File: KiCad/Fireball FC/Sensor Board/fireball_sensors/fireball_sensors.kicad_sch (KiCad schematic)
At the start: 28 parts, among them CN1 HDGC2001WR-S-2P, J1 Conn_01x07, SW2 MAIN POWER, U2 MAX17048G, U3 TPS61023, U5 NCP708, U8 LSM6DSO, U9 MS5607-02BA

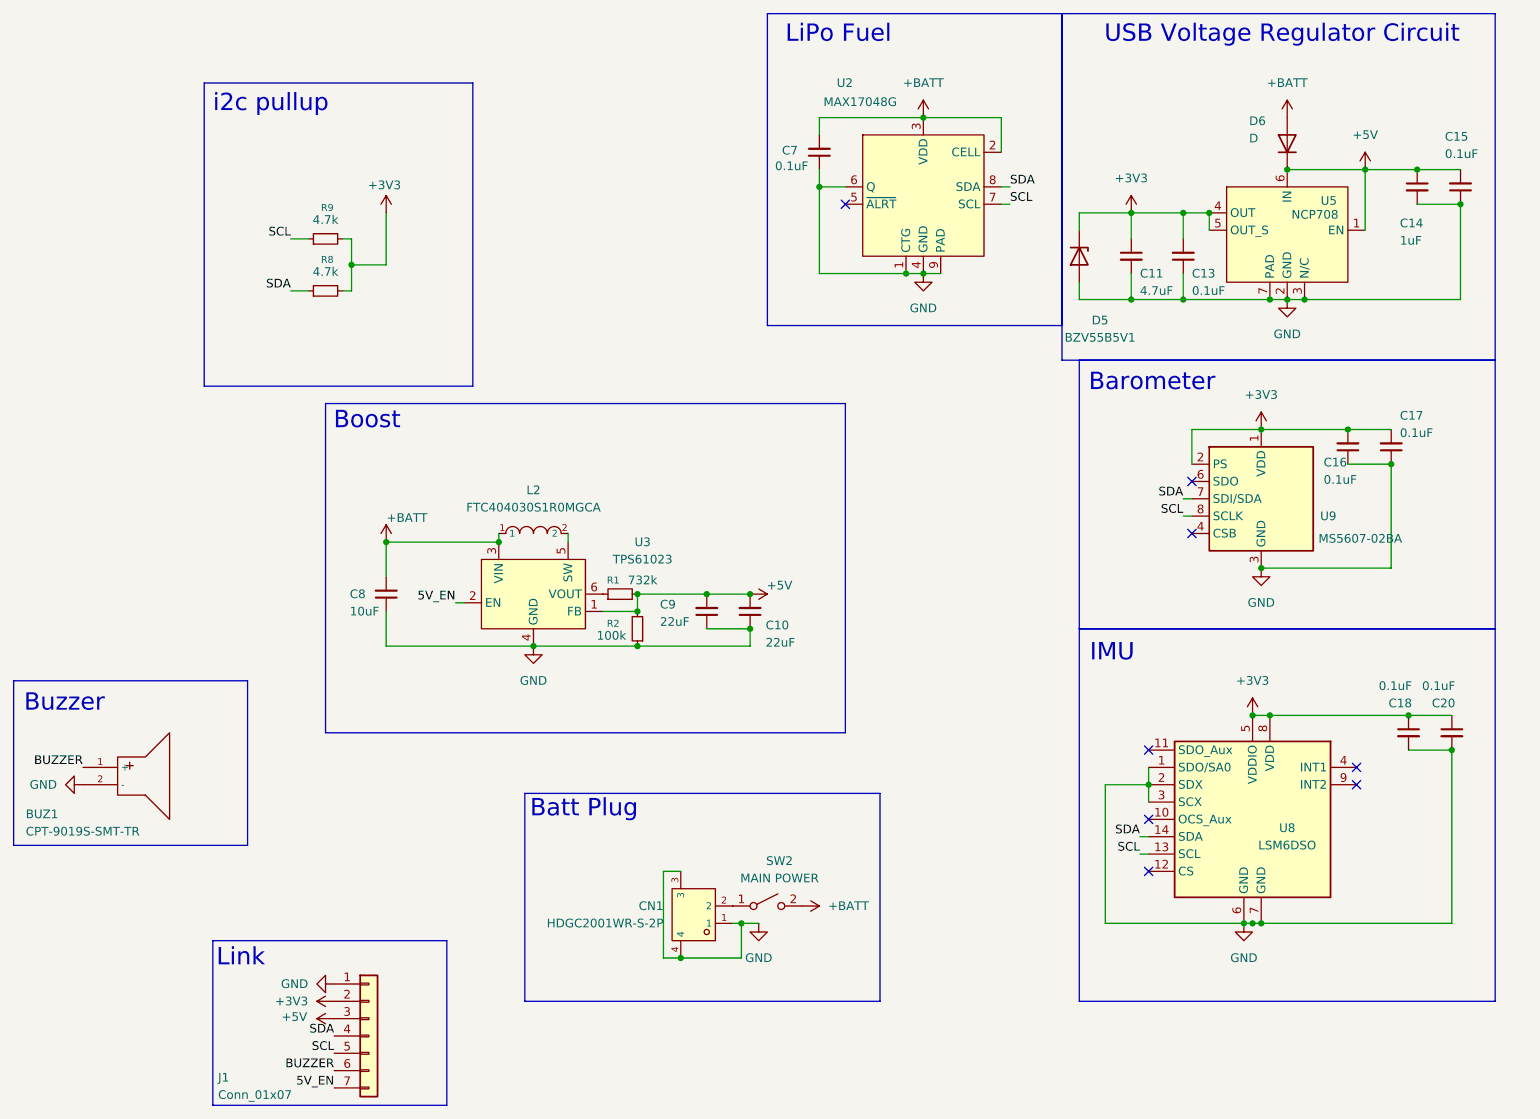
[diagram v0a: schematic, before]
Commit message: routing :D (help)
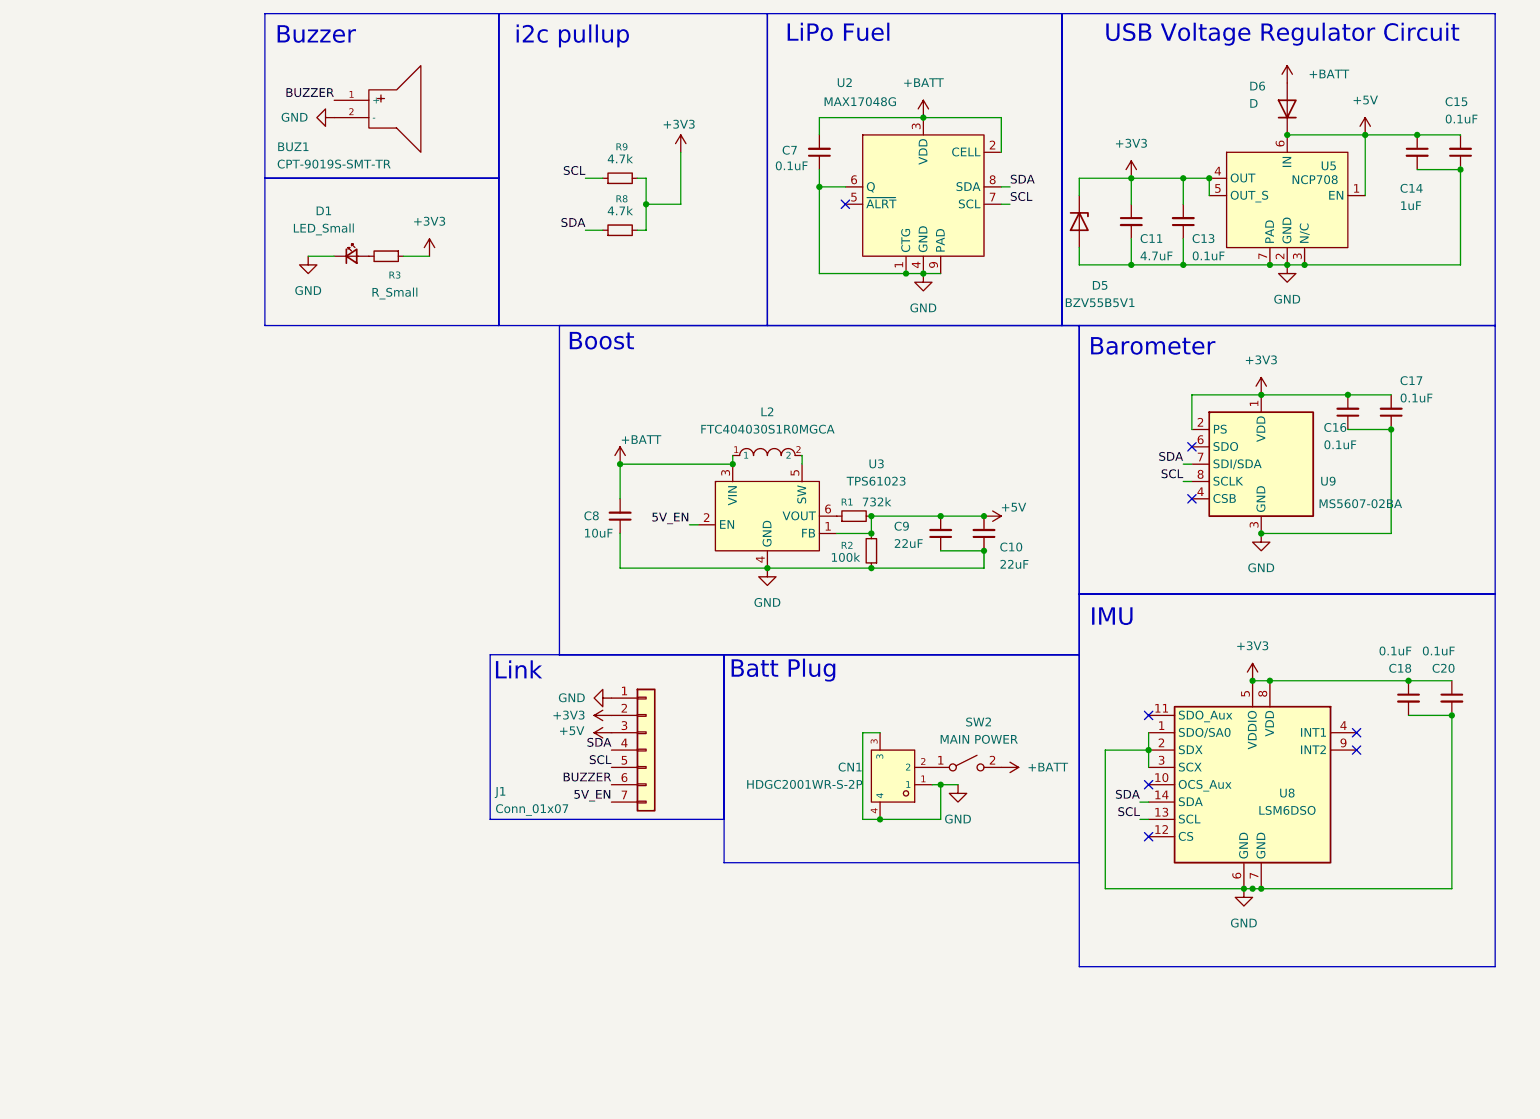
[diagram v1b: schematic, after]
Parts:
- added D1: LED_Small, LED_SMD:LED_0805_2012Metric, symbol Device:LED_Small
- added R3: R_Small, Resistor_SMD:R_0402_1005Metric, symbol Device:R_Small
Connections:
- net +3V3: now also R3.1
- net GND: now also D1.1 (K)
- new net: D1.2 (A), R3.2
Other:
- moved on the sheet: BUZ1, C10, C11, C13, C14, C15, C16, C17, C18, C20, C8, C9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
